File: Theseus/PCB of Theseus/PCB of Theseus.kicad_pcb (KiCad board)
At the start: 2 copper layers, 135 x 80 mm, 127 parts, among them J1 TB001-500-04BE, J11 TB002-500-02BE, J12 TB002-500-02BE, J2 TB001-500-04BE, J3 TB002-500-02BE, J4 TB003-500-P06BE, J5 CN4 STDC14 (Programmer), J6 Micro SD Holder 0472192001, J7 TB002-500-02BE, J8 TB003-500-P06BE, Q1 DMG1012UW-7, Q2 DMG1012UW-7, U1 TPS565201DDC, U11 INA326, U12 INA326, U13 MAX6675, U2 MCP2562, U3 INA326, U4 INA326, U5 MX25L25645G, U6 STM32H750VBTx, Y1 ASE-4.000MHz-L-C-T

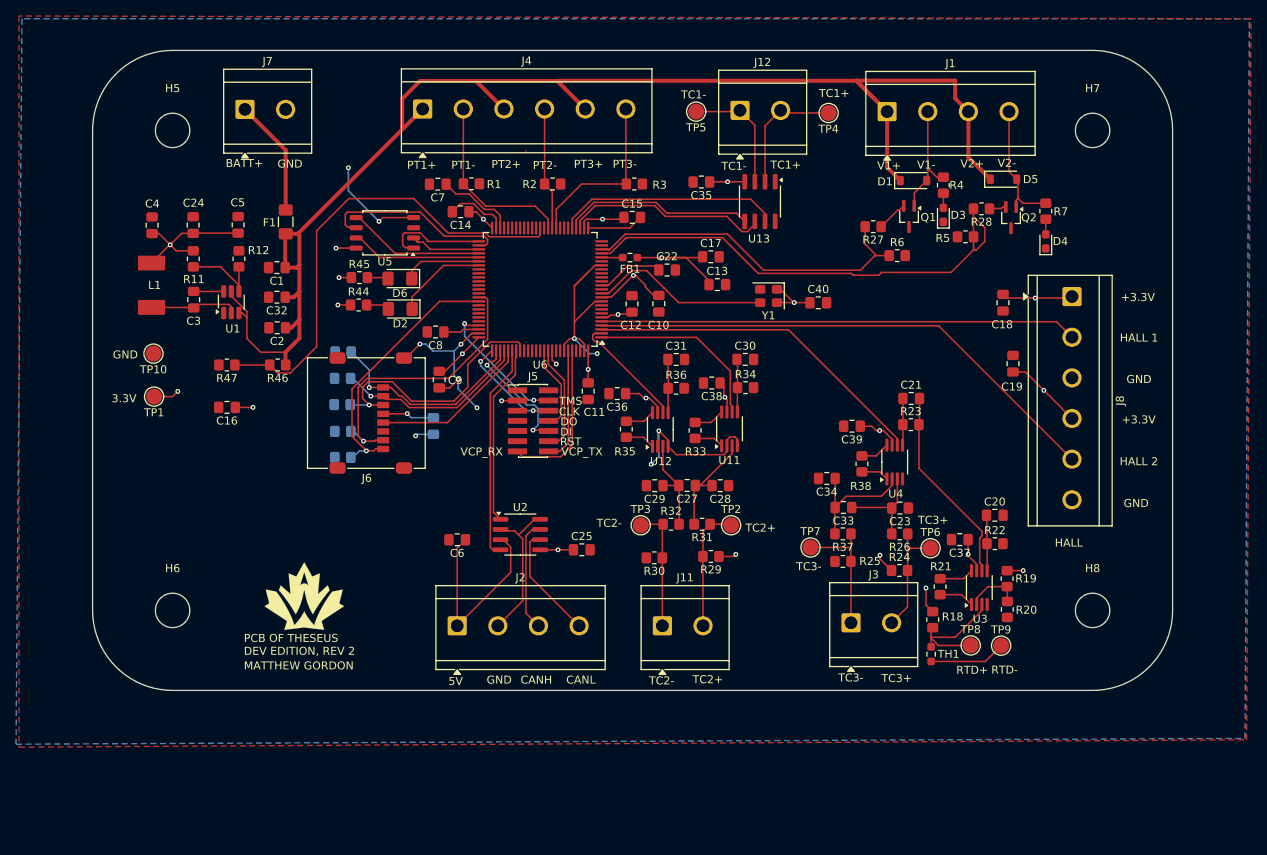
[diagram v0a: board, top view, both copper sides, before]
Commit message: Flight design, first pass
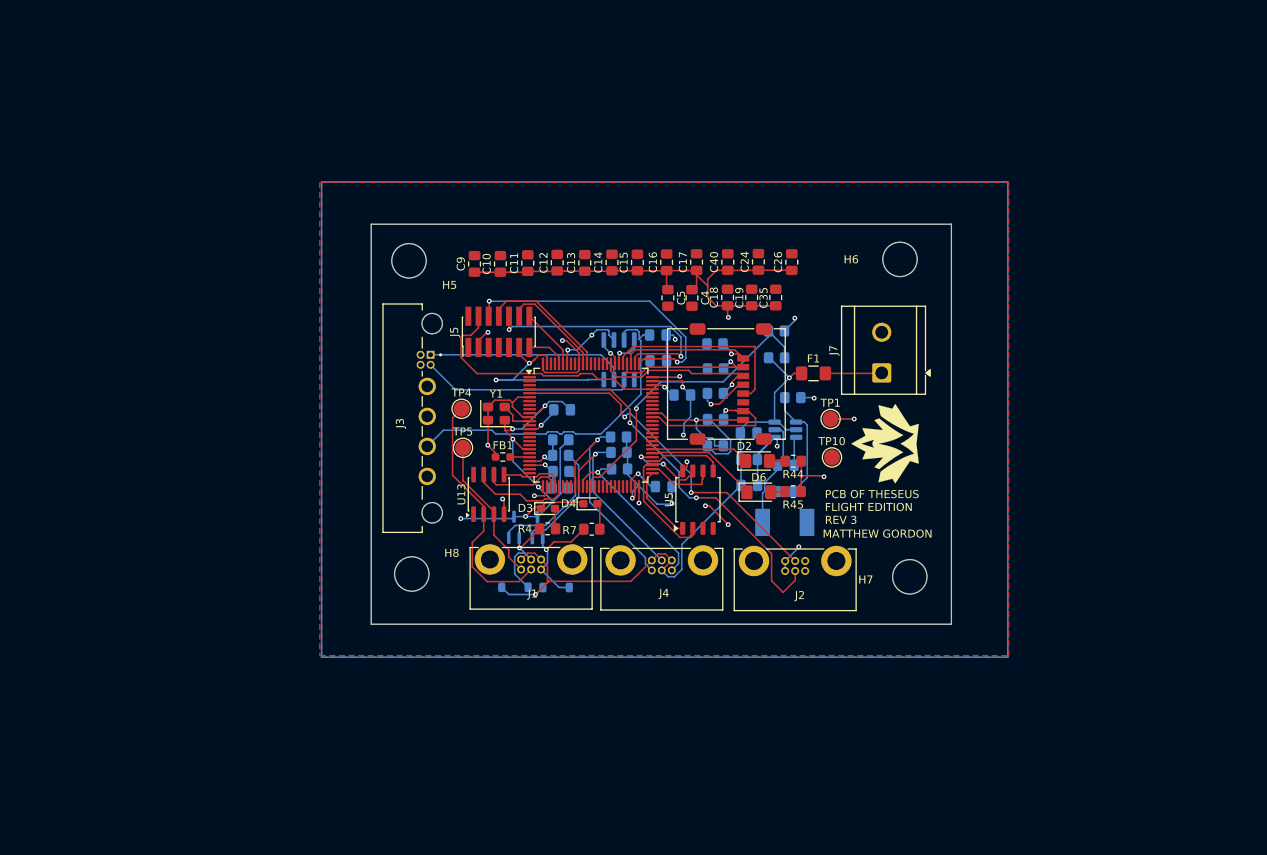
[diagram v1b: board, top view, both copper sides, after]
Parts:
- removed C20, C21: 0.5n, Capacitor_SMD:C_0805_2012Metric_Pad1.18x1.45mm_HandSolder
- removed C23, C28, C29, C34: 0.47u, Capacitor_SMD:C_0805_2012Metric_Pad1.18x1.45mm_HandSolder
- removed C27, C33: 0.047u, Capacitor_SMD:C_0805_2012Metric_Pad1.18x1.45mm_HandSolder
- removed C30, C31: 2n, Capacitor_SMD:C_0805_2012Metric_Pad1.18x1.45mm_HandSolder
- removed C36, C37, C38, C39: 0.1u, Capacitor_SMD:C_0805_2012Metric_Pad1.18x1.45mm_HandSolder
- removed J11, J12: TB002-500-02BE, TerminalBlock_CUI:TerminalBlock_CUI_TB007-508-02_1x02_P5.08mm_Horizontal
- removed J8: TB003-500-P06BE, TerminalBlock_CUI:TerminalBlock_CUI_TB007-508-06_1x06_P5.08mm_Horizontal
- removed R18, R19: 32.4k ±0.1%, Resistor_SMD:R_0805_2012Metric_Pad1.20x1.40mm_HandSolder
- removed R20: 100R ±0.1%, Resistor_SMD:R_0805_2012Metric_Pad1.20x1.40mm_HandSolder
- removed R21, R38: 8.06k, Resistor_SMD:R_0805_2012Metric_Pad1.20x1.40mm_HandSolder
- removed R22, R23: 200k, Resistor_SMD:R_0805_2012Metric_Pad1.20x1.40mm_HandSolder
- removed R24, R25, R30: 1M ±0.1%, Resistor_SMD:R_0805_2012Metric_Pad1.20x1.40mm_HandSolder
- removed R26, R31, R32, R37: 806R, Resistor_SMD:R_0805_2012Metric_Pad1.20x1.40mm_HandSolder
- removed R29: 10M ±1%, Resistor_SMD:R_0805_2012Metric_Pad1.20x1.40mm_HandSolder
- removed R33, R35: 20k, Resistor_SMD:R_0805_2012Metric_Pad1.20x1.40mm_HandSolder
- removed R34, R36: 80.6k, Resistor_SMD:R_0805_2012Metric_Pad1.20x1.40mm_HandSolder
- removed TH1: PTS060301B100RP100, Resistor_SMD:R_0603_1608Metric_Pad0.98x0.95mm_HandSolder
- removed TP2: TC2+, TestPoint:TestPoint_Pad_D2.0mm
- removed TP3: TC2-, TestPoint:TestPoint_Pad_D2.0mm
- removed TP6: TC3+, TestPoint:TestPoint_Pad_D2.0mm
- removed TP7: TC3-, TestPoint:TestPoint_Pad_D2.0mm
- removed TP8: RTD1, TestPoint:TestPoint_Pad_D2.0mm
- removed TP9: RTD2, TestPoint:TestPoint_Pad_D2.0mm
- removed U11, U12, U3, U4: INA326, Package_SO:MSOP-8_3x3mm_P0.65mm
- C1, C2, C22, C25, C3, C32, C6, C7, C8, D1, D5, L1, Q1, Q2, R1, R11, R12, R2, R27, R28, R3, R46, R47, R5, R6, U1, U2: moved to B.Cu
- C26: moved to F.Cu
- J1, J2: value TB001-500-04BE -> Conn_01x06_Socket; footprint TerminalBlock_CUI:TerminalBlock_CUI_TB007-508-04_1x04_P5.08mm_Horizontal -> canhw_footprints:connector_Harwin_G125–MG10605M4P
- J3: value TB002-500-02BE -> G125-MH104M4-04AD000P; footprint TerminalBlock_CUI:TerminalBlock_CUI_TB007-508-02_1x02_P5.08mm_Horizontal -> canhw_footprints:connector_Harwin_G125-MH104M4-04AD000P
- J4: value TB003-500-P06BE -> Conn_01x06_Socket; footprint TerminalBlock_CUI:TerminalBlock_CUI_TB007-508-06_1x06_P5.08mm_Horizontal -> canhw_footprints:connector_Harwin_G125–MG10605M4P
- R13, R14, R15, R16, R17: value 50k -> 51k
- moved H6 101.0 mm to (184.3, 49.8)
- moved J7 86.1 mm to (182.0, 64.0), turned to 90 degrees
- moved TP10 85.8 mm to (175.8, 74.5), turned to 0 degrees
- moved H8 85.2 mm to (123.2, 89.1)
- moved TP1 84.6 mm to (175.6, 69.8), turned to 0 degrees
- moved L1 84.5 mm to (169.9, 82.7), turned to 180 degrees
- moved R11 79.5 mm to (169.9, 78.8), turned to 0 degrees
- moved C3 76.9 mm to (170.0, 75.5), turned to 0 degrees
- moved D5 75.7 mm to (141.3, 90.8)
- moved G*** 75.1 mm to (182.4, 72.8), turned to 90 degrees
- moved J1 71.5 mm to (138.2, 87.3)
- moved R12 71.4 mm to (170.9, 67.1), turned to 0 degrees
- moved D1 71.2 mm to (136.1, 90.8)
- moved U1 71.1 mm to (169.9, 71.1), turned to 0 degrees
- moved C24 70.8 mm to (166.6, 50.1)
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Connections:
- J2 pad 1: +5V -> +3.3V
- J2 pad 2: GND -> /MCU/HALL_1
- J2 pad 3: /CANH -> GND
- J2 pad 4: /CANL -> +3.3V
- J3 pad 1: Net-(J3-Pin_1) -> /CANH
- J3 pad 2: Net-(J3-Pin_2) -> /CANL
- TP4 pad 1: Net-(J12-Pin_2) -> /Valves and Sensors/TC1+
- TP5 pad 1: Net-(J12-Pin_1) -> /Valves and Sensors/TC1-
- U13 pad 2: Net-(J12-Pin_2) -> /Valves and Sensors/TC1+
- U13 pad 3: Net-(J12-Pin_1) -> /Valves and Sensors/TC1-
- U6 pad 1: /MCU/TC2+ -> unconnected-(U6-PE2-Pad1)
- U6 pad 2: /MCU/TC2- -> unconnected-(U6-PE3-Pad2)
- U6 pad 3: /MCU/TC3 -> unconnected-(U6-PE4-Pad3)
- U6 pad 35: /MCU/PT_2 -> /MCU/PT_1
- U6 pad 36: /MCU/PT_1 -> /MCU/PT_2
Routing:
- net +BATT: track 180.9 -> 76.7 mm, vias 0 -> 2
- net /MCU/VALVE_2: track 61.2 -> 5.38 mm, vias 0 -> 1
- net /MCU/TC3: track 43.4 -> 0.00 mm
- net /MCU/VALVE_1: track 43.7 -> 5.40 mm, vias 0 -> 1
- net /Valves and Sensors/TC1+: track 0.00 -> 31.3 mm
- net Net-(C21-Pad2): track 25.1 -> 0.00 mm
- net /MCU/TCK: track 13.4 -> 37.4 mm
- net +3.3V: track 152.3 -> 128.5 mm, vias 29 -> 14
- net /MCU/TC2+: track 23.0 -> 0.00 mm
- net /MCU/V_BATT: track 60.7 -> 37.8 mm, vias 0 -> 1
- net /CAN_Rx: track 27.1 -> 4.45 mm, vias 0 -> 1
- net GND: track 128.5 -> 148.5 mm, vias 11 -> 19
- net /CAN_Tx: track 22.6 -> 3.60 mm, vias 0 -> 1
- net /MCU/OSC_IN: track 22.7 -> 4.25 mm
- net /Valves and Sensors/TC1-: track 0.00 -> 18.2 mm
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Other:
- board size 135 x 80 mm -> 72.5 x 50 mm
- board text added: "PCB OF THESEUS FLIGHT EDITION REV 3"
- board text removed: "+3.3V"
- board text removed: "3.3V"
- board text removed: "5V"
- board text removed: "BATT+"
- board text removed: "CANH"
- board text removed: "CANL"
- board text removed: "CLK"
- board text removed: "DI"
- board text removed: "DO"
- board text removed: "GND"
- board text removed: "HALL"
- board text removed: "HALL 1"
- board text removed: "HALL 2"
- board text removed: "IF YOU'RE READING THIS THE PCB IS UPSIDE-DOWN (OR YOU'RE IN THE SHADOW REALM)"
- board text removed: "PCB OF THESEUS DEV EDITION, REV 2"
- board text removed: "PT1+"
- board text removed: "PT1-"
- board text removed: "PT2+"
- board text removed: "PT2-"
- board text removed: "PT3+"
- board text removed: "PT3-"
- board text removed: "RST"
- board text removed: "RTD+"
- board text removed: "RTD-"
- board text removed: "TC1+"
- board text removed: "TC1-"
- board text removed: "TC2+"
- board text removed: "TC2-"
- board text removed: "TC3+"
- board text removed: "TC3-"
- board text removed: "TMS"
- board text removed: "V1+"
- board text removed: "V1-"
- board text removed: "V2+"
- board text removed: "V2-"
- board text removed: "VCP_RX"
- board text removed: "VCP_TX"

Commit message: Flight design v1
First pass at flight design
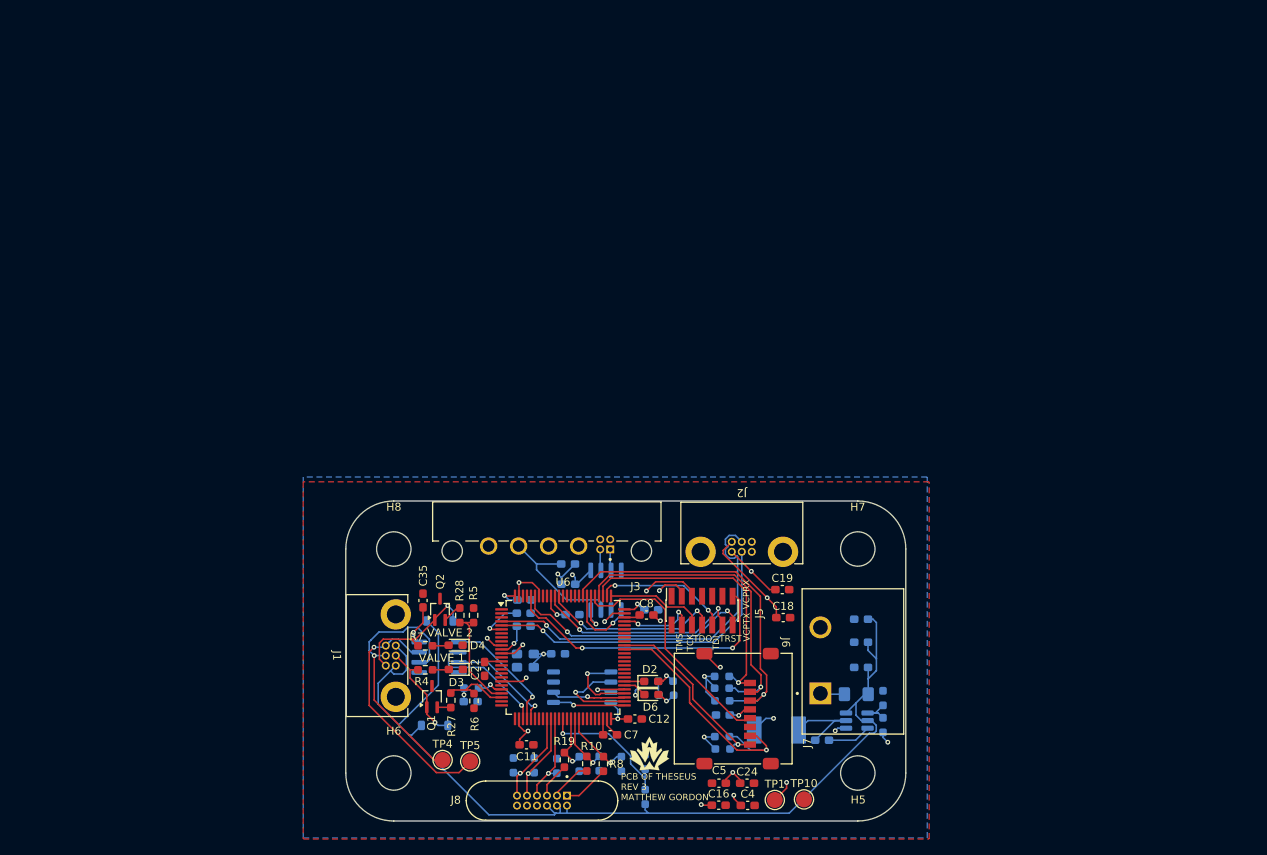
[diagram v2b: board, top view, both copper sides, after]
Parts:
- removed the G*** at (182.4, 72.8)
- removed the G*** at (152.1, 50.5)
- removed J4: Conn_01x06_Socket, canhw_footprints:connector_Harwin_G125–MG10605M4P
- added G***: LOGO, Team_Logo:Logo_SilkScreen_5mm, F.Cu at (152.9, 111.5)
- added J8: Conn_01x12_Socket, canhw_footprints:connector_Harwin_G125-MV11205M1P, F.Cu at (139.5, 117.5)
- added R10: 82K, Resistor_SMD:R_0603_1608Metric_Pad0.98x0.95mm_HandSolder, F.Cu at (145.1, 112.8)
- added R18: 130K, Resistor_SMD:R_0603_1608Metric_Pad0.98x0.95mm_HandSolder, B.Cu at (146.7, 112.8)
- added R19: 82K, Resistor_SMD:R_0603_1608Metric_Pad0.98x0.95mm_HandSolder, F.Cu at (142.3, 112.4)
- added R20: 130K, Resistor_SMD:R_0603_1608Metric_Pad0.98x0.95mm_HandSolder, B.Cu at (144.2, 112.9)
- added R8: 82K, Resistor_SMD:R_0603_1608Metric_Pad0.98x0.95mm_HandSolder, F.Cu at (147.2, 112.9)
- added R9: 130K, Resistor_SMD:R_0603_1608Metric_Pad0.98x0.95mm_HandSolder, B.Cu at (149.4, 112.9)
- C1, C11, C12, C16, C18, C19, C2, C24, C25, C3, C32, C35, C4, C5, C6: footprint Capacitor_SMD:C_0805_2012Metric_Pad1.18x1.45mm_HandSolder -> Capacitor_SMD:C_0603_1608Metric_Pad1.08x0.95mm_HandSolder
- C10, C13, C14, C15, C17, C26, C40, C9: footprint Capacitor_SMD:C_0805_2012Metric_Pad1.18x1.45mm_HandSolder -> Capacitor_SMD:C_0603_1608Metric_Pad1.08x0.95mm_HandSolder; moved to B.Cu
- C22, C7, C8: footprint Capacitor_SMD:C_0805_2012Metric_Pad1.18x1.45mm_HandSolder -> Capacitor_SMD:C_0603_1608Metric_Pad1.08x0.95mm_HandSolder; moved to F.Cu
- D2, D6: footprint Diode_SMD:D_1206_3216Metric_Pad1.42x1.75mm_HandSolder -> Diode_SMD:D_0603_1608Metric_Pad1.05x0.95mm_HandSolder
- F1, FB1, U13, U5, Y1: moved to B.Cu
- J5: footprint Connector_PinHeader_1.27mm:PinHeader_2x07_P1.27mm_Vertical_SMD -> Connector_PinSocket_1.27mm:PinSocket_2x07_P1.27mm_Vertical_SMD
- J7: value TB002-500-02BE -> 4DB-P108-02; footprint TerminalBlock_CUI:TerminalBlock_CUI_TB007-508-02_1x02_P5.08mm_Horizontal -> canhw_footprints:4DB-P108-02
- Q1, Q2: moved to F.Cu
- R1, R11, R12, R13, R14, R15, R16, R17, R2, R3, R4, R7: footprint Resistor_SMD:R_0805_2012Metric_Pad1.20x1.40mm_HandSolder -> Resistor_SMD:R_0603_1608Metric_Pad0.98x0.95mm_HandSolder
- R27, R28, R5, R6: footprint Resistor_SMD:R_0805_2012Metric_Pad1.20x1.40mm_HandSolder -> Resistor_SMD:R_0603_1608Metric_Pad0.98x0.95mm_HandSolder; moved to F.Cu
- R44, R45: footprint Resistor_SMD:R_0805_2012Metric_Pad1.20x1.40mm_HandSolder -> Resistor_SMD:R_0603_1608Metric_Pad0.98x0.95mm_HandSolder; moved to B.Cu
- R46: value 3M ±1% -> 300K; footprint Resistor_SMD:R_0805_2012Metric_Pad1.20x1.40mm_HandSolder -> Resistor_SMD:R_0603_1608Metric_Pad0.98x0.95mm_HandSolder
- R47: value 1M ±0.1% -> 100K; footprint Resistor_SMD:R_0805_2012Metric_Pad1.20x1.40mm_HandSolder -> Resistor_SMD:R_0603_1608Metric_Pad0.98x0.95mm_HandSolder
- moved H6 90.1 mm to (121.0, 114.0)
- moved H5 85.1 mm to (179.0, 114.0)
- moved C16 68.2 mm to (161.6, 118.0), turned to 0 degrees
- moved C24 65.2 mm to (165.2, 115.3), turned to 0 degrees
- moved C4 63.8 mm to (165.2, 118.0), turned to 0 degrees
- moved C17 61.8 mm to (130.6, 105.1), turned to 0 degrees
- moved C5 61.0 mm to (161.6, 115.3), turned to 180 degrees
- moved C11 60.2 mm to (137.6, 110.5), turned to 0 degrees
- moved C35 58.1 mm to (124.7, 92.4)
- moved C12 57.9 mm to (151.1, 107.2), turned to 0 degrees
- moved R46 57.3 mm to (152.4, 117.0), turned to 90 degrees
- moved C26 57.3 mm to (162.1, 106.8), turned to 180 degrees
- moved R47 56.3 mm to (152.4, 112.6), turned to 90 degrees
- moved C40 53.4 mm to (141.5, 99.1), turned to 0 degrees
- moved TP1 48.1 mm to (168.6, 117.4)
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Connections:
- net /MCU/PT_3 renamed /Valves and Sensors/PT3_OUT
- R1 pad 1: /MCU/PT_1 -> /Valves and Sensors/PT1_OUT
- R2 pad 1: /MCU/PT_2 -> /Valves and Sensors/PT2_OUT
- U6 pad 35: /MCU/PT_1 -> /Valves and Sensors/PT2_OUT
- U6 pad 36: /MCU/PT_2 -> /Valves and Sensors/PT1_OUT
- U6 pad 40: unconnected-(U6-PE10-Pad40) -> /MCU/PT6
- U6 pad 41: unconnected-(U6-PE11-Pad41) -> /MCU/PT5
- U6 pad 42: unconnected-(U6-PE12-Pad42) -> /MCU/PT4
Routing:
- net GND: track 148.5 -> 34.1 mm, vias 19 -> 9
- net +BATT: track 76.7 -> 130.2 mm, vias 2 -> 0
- net /MCU/VCP_RX: track 5.05 -> 36.8 mm, vias 0 -> 2
- net +3.3V: track 128.5 -> 100.5 mm, vias 14 -> 24
- net /MCU/TCK: track 37.4 -> 12.3 mm, vias 2 -> 0
- net +5V: track 42.8 -> 17.7 mm
- net /CANL: track 26.6 -> 2.66 mm
- net /MCU/PT_1: track 23.9 -> 0.00 mm, vias 1 -> 0
- net /MCU/VCP_TX: track 7.69 -> 30.9 mm, vias 0 -> 2
- net /MCU/TMS: track 32.4 -> 9.97 mm, vias 0 -> 2
- net /CANH: track 25.1 -> 2.67 mm
- net /MCU/SD_CMD: track 22.4 -> 44.6 mm
- net /MCU/PT_2: track 21.8 -> 0.00 mm, vias 1 -> 0
- net /MCU/SD_D3: track 19.0 -> 40.2 mm
- net /MCU/V_BATT: track 37.8 -> 17.6 mm
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- added copper zone on In2.Cu, net +3.3V
- added copper zone on B.Cu, net GND
- added copper zone on In1.Cu, net GND
- removed copper zone on B.Cu, net +3.3V
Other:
- board size 72.5 x 50 mm -> 70 x 40 mm
- copper layers 2 -> 4
- board text added: "PCB OF THESEUS REV 3 MATTHEW GORDON"
- board text added: "TCK"
- board text added: "TDI"
- board text added: "TDO"
- board text added: "TMS"
- board text added: "TRST"
- board text added: "VALVE 1"
- board text added: "VALVE 2"
- board text added: "VCPRX"
- board text added: "VCPTX"
- board text removed: "MATTHEW GORDON"
- board text removed: "PCB OF THESEUS FLIGHT EDITION REV 3"
